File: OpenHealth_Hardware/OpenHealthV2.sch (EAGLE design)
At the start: 21 parts

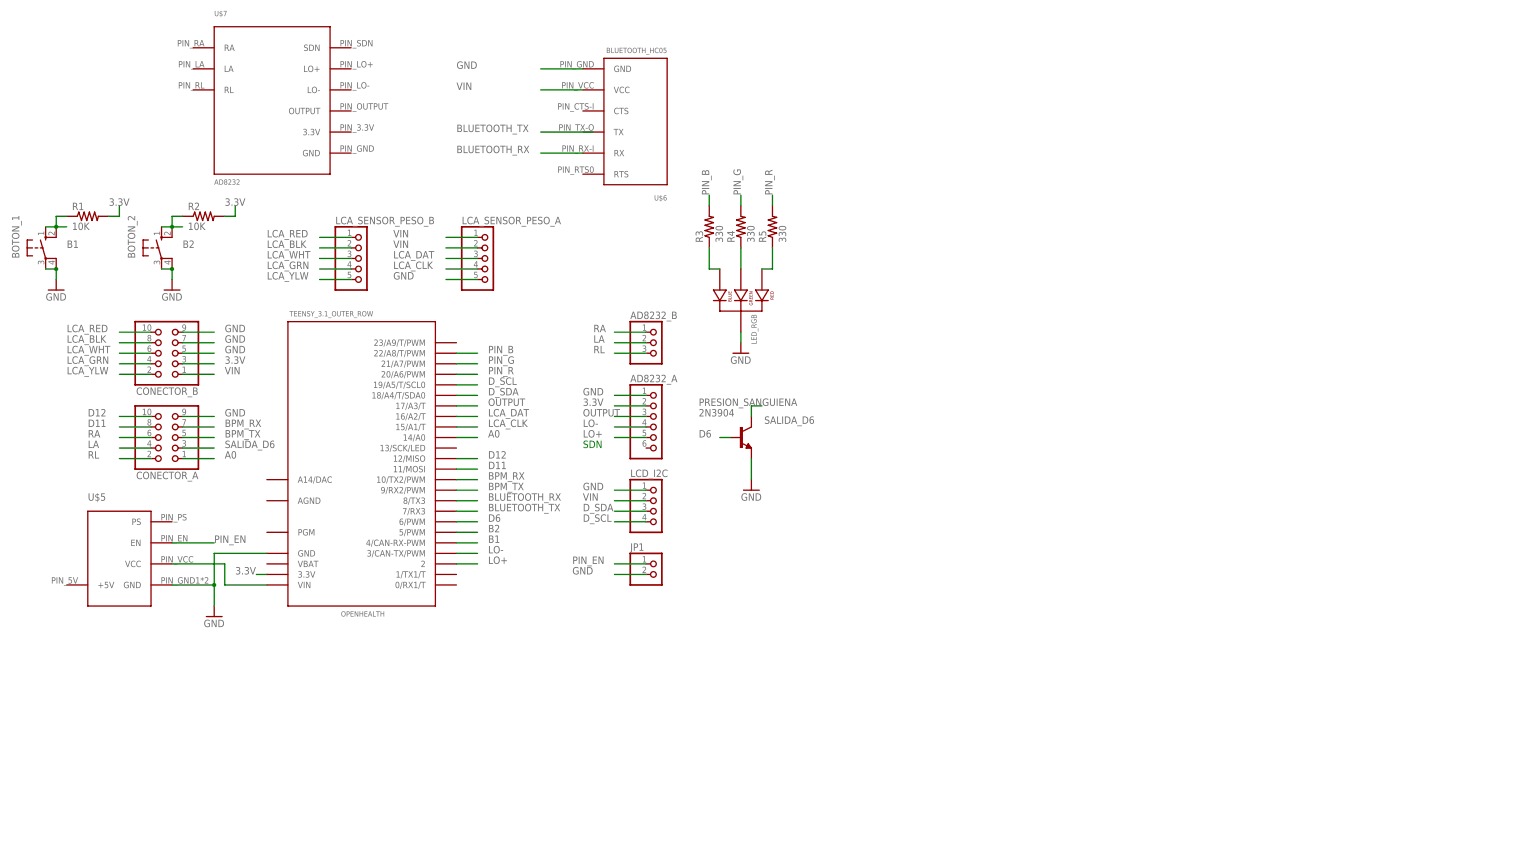
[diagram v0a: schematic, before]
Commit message: Finalizacion de la primera version, listo para revision
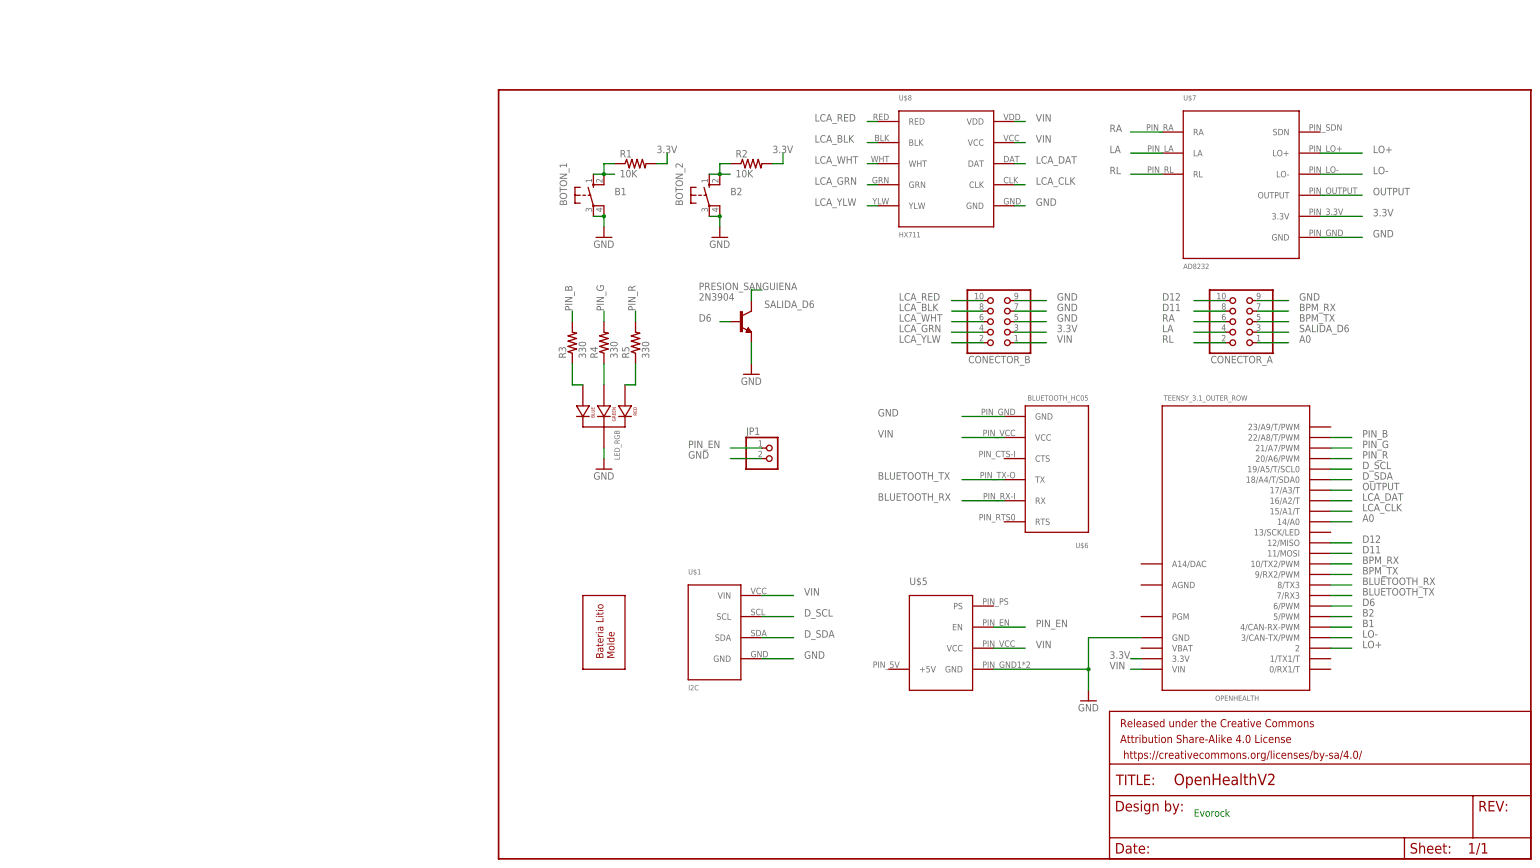
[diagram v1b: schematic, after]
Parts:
- removed AD8232_A: (no value), pinhead:PINHD-1X6
- removed AD8232_B: (no value), pinhead:PINHD-1X3
- removed LCA_SENSOR_PESO_A, LCA_SENSOR_PESO_B: (no value), pinhead:PINHD-1X5
- removed LCD_I2C: (no value), pinhead:PINHD-1X4
- added FRAME1: FRAME-LETTER, SparkFun-Aesthetics:FRAME-LETTER
- added U$1: I2C, OpenHealth:I2C
- added U$2: BATERRY_MOLD, OpenHealth:BATERRY_MOLD
- added U$8: HX711, OpenHealth:HX711
- BOTON_1, BOTON_2, CONECTOR_A, CONECTOR_B, JP1: value (none) -> (none)
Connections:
- removed net N$5: OPENHEALTH.VIN, U$5.VCC
- net 3.3V: now also U$7.3.3V; no longer AD8232_A.2
- net BLUETOOTH_TX: now also U$6.TX
- net D_SCL: now also U$1.SCL; no longer LCD_I2C.4
- net D_SDA: now also U$1.SDA; no longer LCD_I2C.3
- net GND: now also U$1.GND, U$7.GND, U$8.GND; no longer AD8232_A.1, LCA_SENSOR_PESO_A.5, LCD_I2C.1
- net LA: now also U$7.LA; no longer AD8232_B.2
- net LCA_BLK: now also U$8.BLK; no longer LCA_SENSOR_PESO_B.2
- net LCA_CLK: now also U$8.CLK; no longer LCA_SENSOR_PESO_A.4
- net LCA_DAT: now also U$8.DAT; no longer LCA_SENSOR_PESO_A.3
- net LCA_GRN: now also U$8.GRN; no longer LCA_SENSOR_PESO_B.4
- net LCA_RED: now also U$8.RED; no longer LCA_SENSOR_PESO_B.1
- net LCA_WHT: now also U$8.WHT; no longer LCA_SENSOR_PESO_B.3
- net LCA_YLW: now also U$8.YLW; no longer LCA_SENSOR_PESO_B.5
- net LO+: now also U$7.LO+; no longer AD8232_A.5
- net LO-: now also U$7.LO-; no longer AD8232_A.4
- net OUTPUT: now also U$7.OUTPUT; no longer AD8232_A.3
- net RA: now also U$7.RA; no longer AD8232_B.1
- net RL: now also U$7.RL; no longer AD8232_B.3
- net VIN: now also OPENHEALTH.VIN, U$1.VIN, U$5.VCC, U$8.VCC, U$8.VDD; no longer LCA_SENSOR_PESO_A.1, LCA_SENSOR_PESO_A.2, LCD_I2C.2
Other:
- note added: "Evorock"
- note removed: "SDN"
- moved on the sheet: BOTON_1, BOTON_2, CONECTOR_A, CONECTOR_B, JP1, LED_RGB, OPENHEALTH, PRESION_SANGUIENA, R1, R2, R3, R4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
